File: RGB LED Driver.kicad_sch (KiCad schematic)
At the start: 4 parts

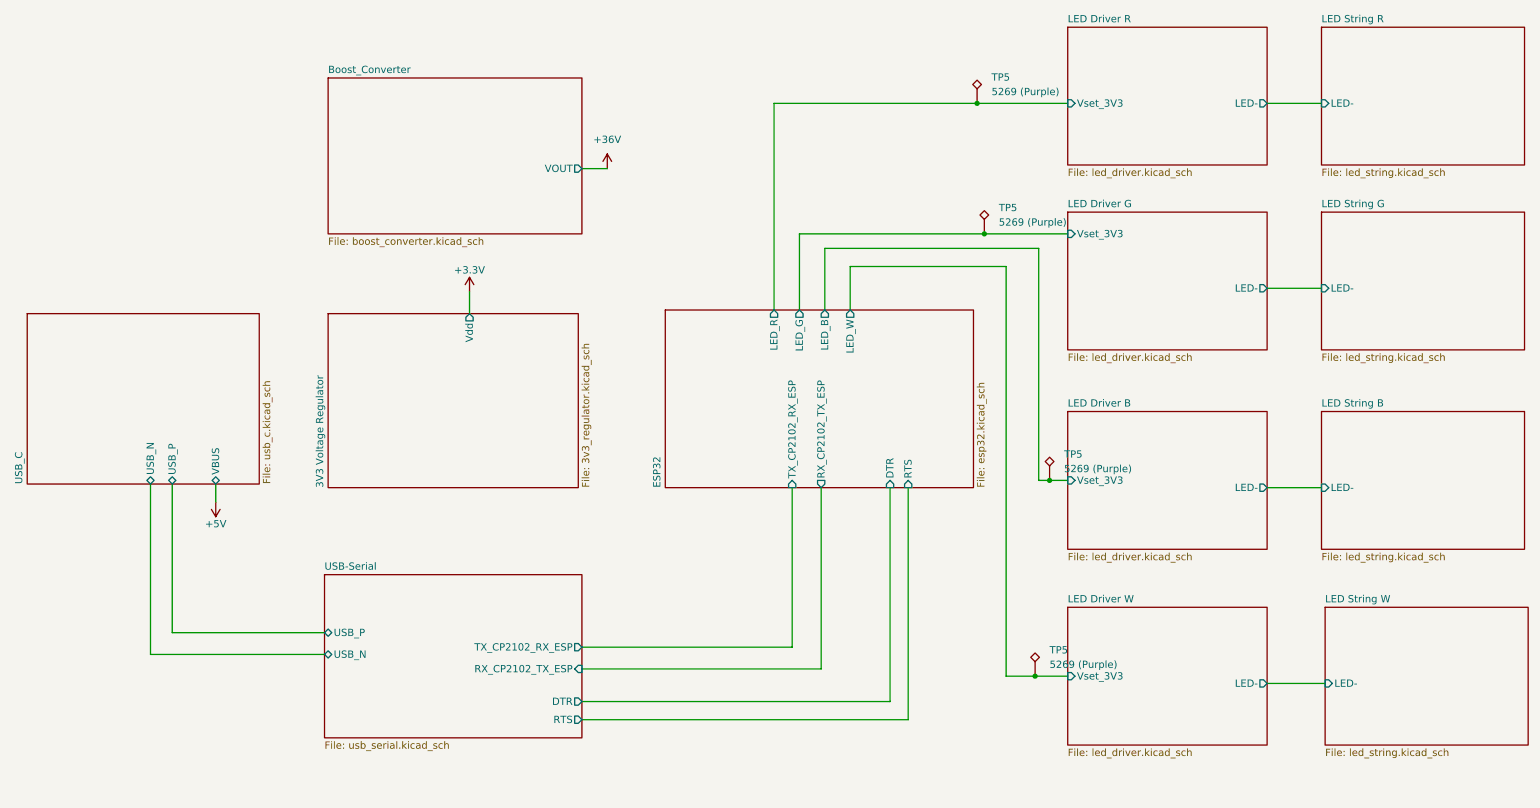
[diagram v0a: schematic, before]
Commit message: neat-ified schematics
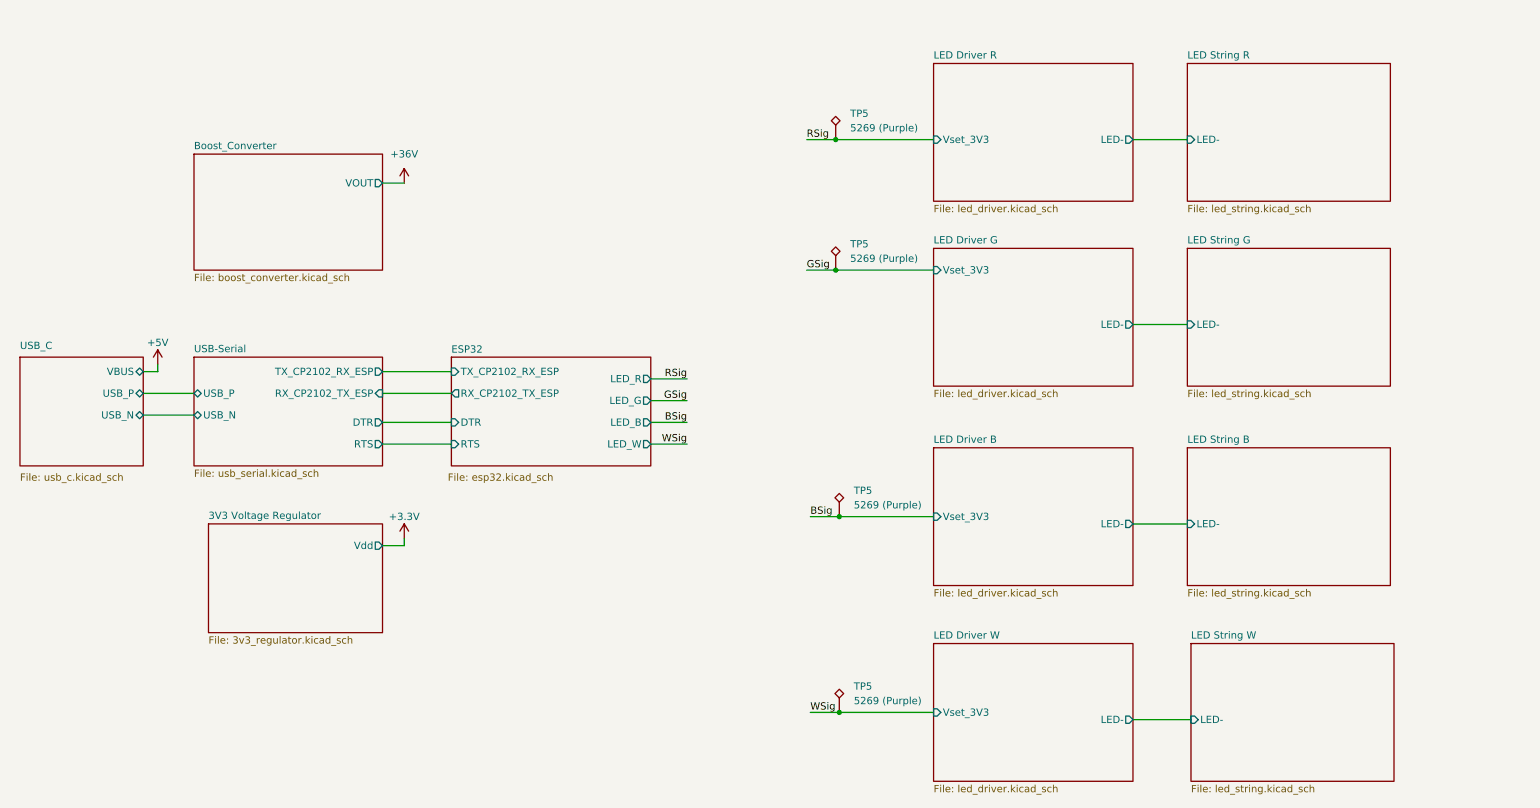
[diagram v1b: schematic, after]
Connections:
- net ESP32/LED_B renamed BSig
- net ESP32/LED_G renamed GSig
- net ESP32/LED_R renamed RSig
- net ESP32/LED_W renamed WSig
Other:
- company: (none) -> The Art and Science of PCB Design
- title: (none) -> RGB LED Driver Demo Board
- moved on the sheet: TP5

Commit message: added digikey PNs
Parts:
- TP5: Digikey PN (none) -> 36-5269-ND; MPN (none) -> 5269
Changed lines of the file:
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@@
       (effects (font (size 1.27 1.27)) hide)
     )
-    (property "Digikey PN" "" (at 159.385 66.04 0)
+    (property "Digikey PN" "36-5269-ND" (at 159.385 66.04 0)
+      (effects (font (size 1.27 1.27)) hide)
+    )
+    (property "MPN" "5269" (at 159.385 66.04 0)
       (effects (font (size 1.27 1.27)) hide)
     )
@@
       (effects (font (size 1.27 1.27)) hide)
     )
-    (property "Digikey PN" "" (at 160.02 143.51 0)
+    (property "Digikey PN" "36-5269-ND" (at 160.02 143.51 0)
+      (effects (font (size 1.27 1.27)) hide)
+    )
+    (property "MPN" "5269" (at 160.02 143.51 0)
       (effects (font (size 1.27 1.27)) hide)
     )
@@
       (effects (font (size 1.27 1.27)) hide)
     )
-    (property "Digikey PN" "" (at 160.02 109.22 0)
+    (property "Digikey PN" "36-5269-ND" (at 160.02 109.22 0)
+      (effects (font (size 1.27 1.27)) hide)
+    )
+    (property "MPN" "5269" (at 160.02 109.22 0)
       (effects (font (size 1.27 1.27)) hide)
     )
@@
       (effects (font (size 1.27 1.27)) hide)
     )
-    (property "Digikey PN" "" (at 159.385 43.18 0)
+    (property "Digikey PN" "36-5269-ND" (at 159.385 43.18 0)
       (effects (font (size 1.27 1.27)) hide)
     )
+    (property "MPN" "5269" (at 159.385 43.18 0)
+      (effects (font (size 1.27 1.27)) hide)
+    )
